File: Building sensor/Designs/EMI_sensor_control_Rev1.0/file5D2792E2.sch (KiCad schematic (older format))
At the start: 31 parts

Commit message: Weekly Push
Weekly Push
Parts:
- removed AE?: Antenna_Loop Bx, symbol Device:Antenna_Loop
- removed AE?: Antenna_Loop Rx, symbol Device:Antenna_Loop
- removed C? (x3): C 0.1u, symbol Device:C_Small
- removed C? (x4): C, symbol Device:C_Small
- removed J?: Conn_01x06_Male, symbol Connector:Conn_01x06_Male
- removed L? (x3): L 1.2u, symbol Device:L
- removed R? (x2): R 22ohm, symbol Device:R
- removed R? (x10): R, symbol Device:R
- removed R? (x3): R 47, symbol Device:R
- removed U? (x2): INA163UA_2K5, D14, symbol 2019-07-16_16-02-38:INA163UA_2K5
- removed U?: ADA4096-2ARMZ, RM_8, symbol 2019-07-11_16-06-15:ADA4096-2ARMZ
- added C62, C63, C64, C65, C66, C73, C74, C75, C76, C78, C79, C80, C81, C82, C83, C84, C85, C86: C 100n, Capacitor_SMD:C_0603_1608Metric_Pad1.05x0.95mm_HandSolder, symbol Device:C
- added C67: C 10u, Capacitor_SMD:C_1210_3225Metric_Pad1.42x2.65mm_HandSolder, symbol Device:C
- added C68, C72: C 1u, Capacitor_SMD:C_0805_2012Metric_Pad1.15x1.40mm_HandSolder, symbol Device:C
- added C69, C70: C 2.2u, Capacitor_SMD:C_0603_1608Metric_Pad1.05x0.95mm_HandSolder, symbol Device:C
- added C71: C 10n, Capacitor_SMD:C_0805_2012Metric_Pad1.15x1.40mm_HandSolder, symbol Device:C
- added C77: C 4.7u, Capacitor_SMD:C_0805_2012Metric_Pad1.15x1.40mm_HandSolder, symbol Device:C
- added CR2: ST3232BDR, symbol 2019-08-01_14-53-54:ST3232BDR
- added J2: Conn_02x07_Odd_Even, Connector_PinHeader_2.54mm:PinHeader_2x07_P2.54mm_Vertical_SMD, symbol Connector_Generic:Conn_02x07_Odd_Even
- added J3: DB9_Female, symbol Connector:DB9_Female
- added R62, R63, R64: R 10k, symbol Device:R
- added SW2: SW_Push, symbol Switch:SW_Push
- added U16: STM32F412ZETx, Package_QFP:LQFP-144_20x20mm_P0.5mm, symbol MCU_ST_STM32F4:STM32F412ZETx
- added Y1: ECS-3963-400-BN-TR, ECS-3963-400-BN-TR:OSC_ECS-3963-400-BN-TR, symbol ECS-3963-400-BN-TR:ECS-3963-400-BN-TR
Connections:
- net +5V: now also Y1.4 (VDD)
- net GND: now also C64.2, C65.1, C66.2, C69.1, C70.1, C73.2, C74.1, C75.1, C76.1, C77.1, C78.1, C79.1, C80.1, C81.1, C82.1, C83.1, C84.1, C85.1, C86.1, CR2.15 (GND), J2.11 (Pin_11), J2.5 (Pin_5), J2.7 (Pin_7), J3.5, R62.2, SW2.2, U16.107 (VSS), U16.120 (VSS), U16.130 (VSS), U16.16 (VSS), U16.38 (VSS), U16.51 (VSS), U16.61 (VSS), U16.83 (VSS), U16.94 (VSS), Y1.2 (GND)
- new net: C62.2, CR2.1 (C1+)
- new net: CR2.13 (R1IN), J3.2
- new net: CR2.14 (T1OUT), J3.3
- new net: C64.1, CR2.2 (V+)
- new net: C62.1, CR2.3 (C1-)
- new net: C63.2, CR2.4 (C2+)
- new net: C63.1, CR2.5 (C2-)
- new net: C65.2, CR2.6 (V-)
- new net: C69.2, U16.106 (VCAP_2)
- new net: C70.2, U16.71 (VCAP_1)
- new net: R63.2, U16.143 (PDR_ON)
- new net: R64.2, U16.138 (BOOT0)
- new net: C73.1, SW2.1, U16.25 (NRST)
- new net: R62.1, U16.48 (PB2)
- new net +3V3: C66.1, C71.2, C72.2, C74.2, C75.2, C76.2, C77.2, C78.2, C79.2, C80.2, C81.2, C82.2, C83.2, C84.2, C85.2, C86.2, CR2.16 (VCC), J2.3 (Pin_3), R63.1, R64.1, U16.108 (VDD), U16.121 (VDD), U16.131 (VDD), U16.144 (VDD), U16.17 (VDD), U16.30 (VDD), U16.33 (VDDA), U16.39 (VDD), U16.52 (VDD), U16.6 (VBAT), U16.62 (VDD), U16.72 (VDD), U16.84 (VDD), U16.95 (VDD_USB)
- new net 5vComm: J3.9
- new net DO_Rx: CR2.12 (R1OUT), U16.97 (PC7)
- new net DO_Tx: CR2.11 (T1IN), U16.96 (PC6)
- new net FPGA_CDONE: U16.37 (PA3)
- new net FPGA_CLK: U16.41 (PA5)
- new net FPGA_Config: U16.36 (PA2)
- new net FPGA_MISO: U16.42 (PA6)
- new net FPGA_MOSI: U16.43 (PA7)
- new net FPGA_SS: U16.40 (PA4)
- new net GNDREF: C67.1, C68.1, C71.1, C72.1, U16.31 (VSSA)
- new net JTCK: J2.6 (Pin_6), J2.9 (Pin_9), U16.109 (PA14)
- new net JTDI: J2.10 (Pin_10), U16.110 (PA15)
- new net JTDO: J2.8 (Pin_8), U16.133 (PB3)
- new net JTMS: J2.4 (Pin_4), U16.105 (PA13)
- new net JTRST: J2.12 (Pin_12), U16.134 (PB4)
- new net MCLK: Y1.3 (OUTPUT)
- new net PWROn: J3.1
- new net TX_On: U16.35 (PA1)
- new net TxC1: U16.100 (PA8)
- new net TxC2: U16.98 (PC8)
- new net VCP_Rx: J2.13 (Pin_13), U16.102 (PA10)
- new net VCP_Tx: J2.14 (Pin_14), U16.101 (PA9)
- new net Vref2.1: C67.2, C68.2, U16.32 (VREF+)
- no-connect marks 4 -> 102

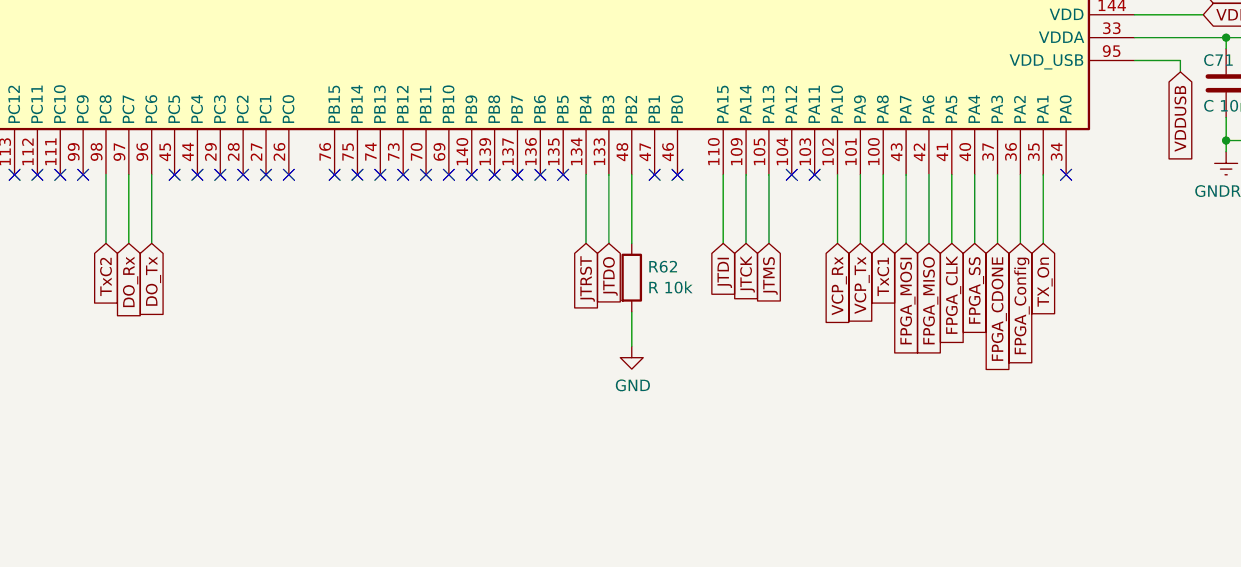
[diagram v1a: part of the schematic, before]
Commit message: Weekly Commit
Weekly Commit 08/09/2019
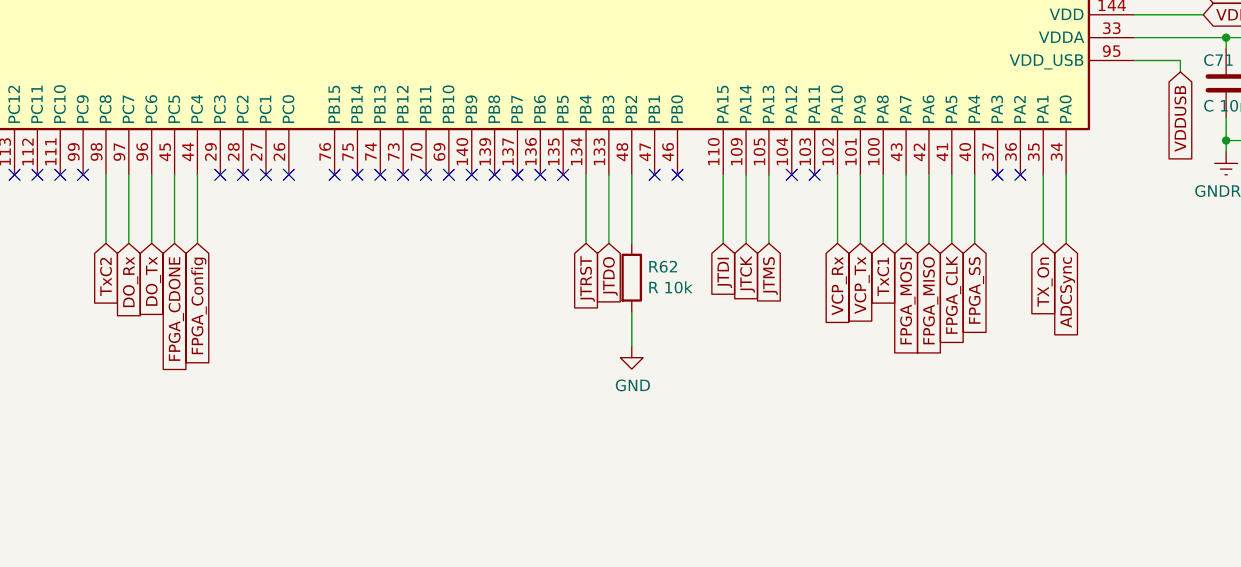
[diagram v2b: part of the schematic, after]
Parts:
- CR2: footprint (none) -> footprints:ST3232BDR
- J3: footprint (none) -> digikey-footprints:DSUB-9_Receptical_A-DF_09_A_KG-T2S
- R62, R63, R64: footprint (none) -> Resistor_SMD:R_1206_3216Metric_Pad1.42x1.75mm_HandSolder
- SW2: footprint (none) -> 1437566-4:SW_1437566-4
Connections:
- net FPGA_CDONE: now also U16.45 (PC5); no longer U16.37 (PA3)
- net FPGA_Config: now also U16.44 (PC4); no longer U16.36 (PA2)
- net ADCSync: now reaches U16.34 (PA0)
- no-connect marks 102 -> 101
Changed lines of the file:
@@
 F 0 "R63" H 11320 3796 50  0000 L CNN
 F 1 "R 10k" H 11320 3705 50  0000 L CNN
-F 2 "" V 11180 3750 50  0001 C CNN
+F 2 "Resistor_SMD:R_1206_3216Metric_Pad1.42x1.75mm_HandSolder" V 11180 3750 50  0001 C CNN
 F 3 "~" H 11250 3750 50  0001 C CNN
 	1    11250 3750
@@
 Text GLabel 10600 6900 3    50   Input ~ 0
 FPGA_CLK
-Text GLabel 10900 6900 3    50   Input ~ 0
+Text GLabel 7300 6900 3    50   Input ~ 0
 FPGA_Config
 Text GLabel 10400 6900 3    50   Input ~ 0
 FPGA_MOSI
-Text GLabel 10800 6900 3    50   Input ~ 0
+Text GLabel 7200 6900 3    50   Input ~ 0
 FPGA_CDONE
 Wire Wire Line
@@
 	10400 6900 10400 6600
 Wire Wire Line
-	10900 6900 10900 6600
-Wire Wire Line
-	10800 6600 10800 6900
+	7300 6900 7300 6600
+Wire Wire Line
+	7200 6600 7200 6900
 Text GLabel 11000 6900 3    50   Input ~ 0
 TX_On
@@
 F 0 "R64" H 11670 3796 50  0000 L CNN
 F 1 "R 10k" H 11670 3705 50  0000 L CNN
-F 2 "" V 11530 3750 50  0001 C CNN
+F 2 "Resistor_SMD:R_1206_3216Metric_Pad1.42x1.75mm_HandSolder" V 11530 3750 50  0001 C CNN
 F 3 "~" H 11600 3750 50  0001 C CNN
 	1    11600 3750
@@
 F 0 "SW2" V 11904 4598 50  0000 L CNN
 F 1 "SW_Push" V 11995 4598 50  0000 L CNN
-F 2 "" H 11950 4650 50  0001 C CNN
+F 2 "1437566-4:SW_1437566-4" H 11950 4650 50  0001 C CNN
 F 3 "~" H 11950 4650 50  0001 C CNN
 	1    11950 4450
@@
 F 0 "R62" H 9270 7096 50  0000 L CNN
 F 1 "R 10k" H 9270 7005 50  0000 L CNN
-F 2 "" V 9130 7050 50  0001 C CNN
+F 2 "Resistor_SMD:R_1206_3216Metric_Pad1.42x1.75mm_HandSolder" V 9130 7050 50  0001 C CNN
 F 3 "~" H 9200 7050 50  0001 C CNN
 	1    9200 7050
@@
 Wire Wire Line
 	9200 7200 9200 7350
-NoConn ~ 11100 6600
 NoConn ~ 10000 6600
 NoConn ~ 9900 6600
@@
 NoConn ~ 7500 6600
 NoConn ~ 7400 6600
-NoConn ~ 7300 6600
-NoConn ~ 7200 6600
 NoConn ~ 6500 6600
 NoConn ~ 6400 6600
@@
 F 0 "CR2" H 4200 9187 60  0000 C CNN
 F 1 "ST3232BDR" H 4200 9081 60  0000 C CNN
-F 2 "" H 4200 9040 60  0001 C CNN
+F 2 "footprints:ST3232BDR" H 4200 9040 60  0001 C CNN
 F 3 "" H 2900 8800 60  0000 C CNN
 	1    2900 8800
@@
 F 0 "J3" H 7268 9842 50  0000 C CNN
 F 1 "DB9_Female" H 7268 9751 50  0000 C CNN
-F 2 "" H 7350 9150 50  0001 C CNN
+F 2 "digikey-footprints:DSUB-9_Receptical_A-DF_09_A_KG-T2S" H 7350 9150 50  0001 C CNN
 F 3 " ~" H 7350 9150 50  0001 C CNN
 	1    7350 9150
@@
 Wire Wire Line
 	2800 8900 2800 8700
+NoConn ~ 10800 6600
+NoConn ~ 10900 6600
+Text GLabel 11100 6900 3    50   Input ~ 0
+ADCSync
+Wire Wire Line
+	11100 6600 11100 6900
 $EndSCHEMATC
